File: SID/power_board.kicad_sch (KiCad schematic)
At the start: 0 parts

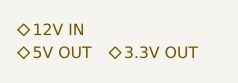
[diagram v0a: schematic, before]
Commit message: Feat(SID): basically complete
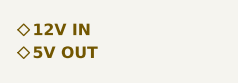
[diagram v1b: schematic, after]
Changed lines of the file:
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@@
-(kicad_sch (version 20230819) (generator eeschema)
-  (paper "A4")
-  (hierarchical_label "5V OUT" (shape bidirectional) (at 109.22 88.9 0) (fields_autoplaced)
-    (effects (font (size 1.27 1.27)) (justify left))
-  )
-  (hierarchical_label "12V IN" (shape bidirectional) (at 109.22 86.36 0) (fields_autoplaced)
-    (effects (font (size 1.27 1.27)) (justify left))
-  )
-  (hierarchical_label "3.3V OUT" (shape bidirectional) (at 119.38 88.9 0) (fields_autoplaced)
-    (effects (font (size 1.27 1.27)) (justify left))
-  )
+(kicad_sch
+	(version 20240101)
+	(generator "eeschema")
+	(generator_version "8.99")
+	(paper "A4")
+	(hierarchical_label "5V OUT"
+		(shape bidirectional)
+		(at 109.22 88.9 0)
+		(fields_autoplaced yes)
+		(effects
+			(font
+				(face "JetBrains Mono")
+				(size 1.27 1.27)
+				(thickness 0.254)
+				(bold yes)
+			)
+			(justify left)
+		)
+	)
+	(hierarchical_label "12V IN"
+		(shape bidirectional)
+		(at 109.22 86.36 0)
+		(fields_autoplaced yes)
+		(effects
+			(font
+				(face "JetBrains Mono")
+				(size 1.27 1.27)
+				(thickness 0.254)
+				(bold yes)
+			)
+			(justify left)
+		)
+	)
 )
